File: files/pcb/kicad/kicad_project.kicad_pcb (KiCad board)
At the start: 2 copper layers, 100 x 102 mm, 115 parts, among them CON1 USB_MINI_B, IC1 ATMEGA328-A, IC10 FET, IC11 DS1307, IC12 LPS331AP, IC13 AM2321, IC2 IC_16PIN, IC3 IC_4PIN, IC4 IC_4PIN, IC5 SN74141_K155NA, IC6 TLP627-4, IC7 TLP627-4, IC8 MY_3_TERMINAL_REGULATOR, IC9 ICM7555CD, K1 CONN_3, K2 CONN_3, K3 CONN_3, K4 CONN_3, P1 CONN_6, SW1 SW_PUSH, SW2 EVQWK, SW3 SW_PUSH, SW4 SW_PUSH, SW5 SW_PUSH, T1 2SC, T2 2SC, T3 2SA, U1 NEON, U10 NIXIE_IN_16, U11 DC_JACK, U12 LOAD, U13 remocon, U14 napion, U15 MY_PIN52, U16 MY_PIN52, U17 MY_PIN52, U18 MY_PIN52, U2 NEON, U3 NEON, U4 NEON, U5 NIXIE_IN_16, U6 NIXIE_IN_16, U7 NIXIE_IN_16, U8 NIXIE_IN_16, U9 NIXIE_IN_16, X1 12MHz, X2 32.768kHz

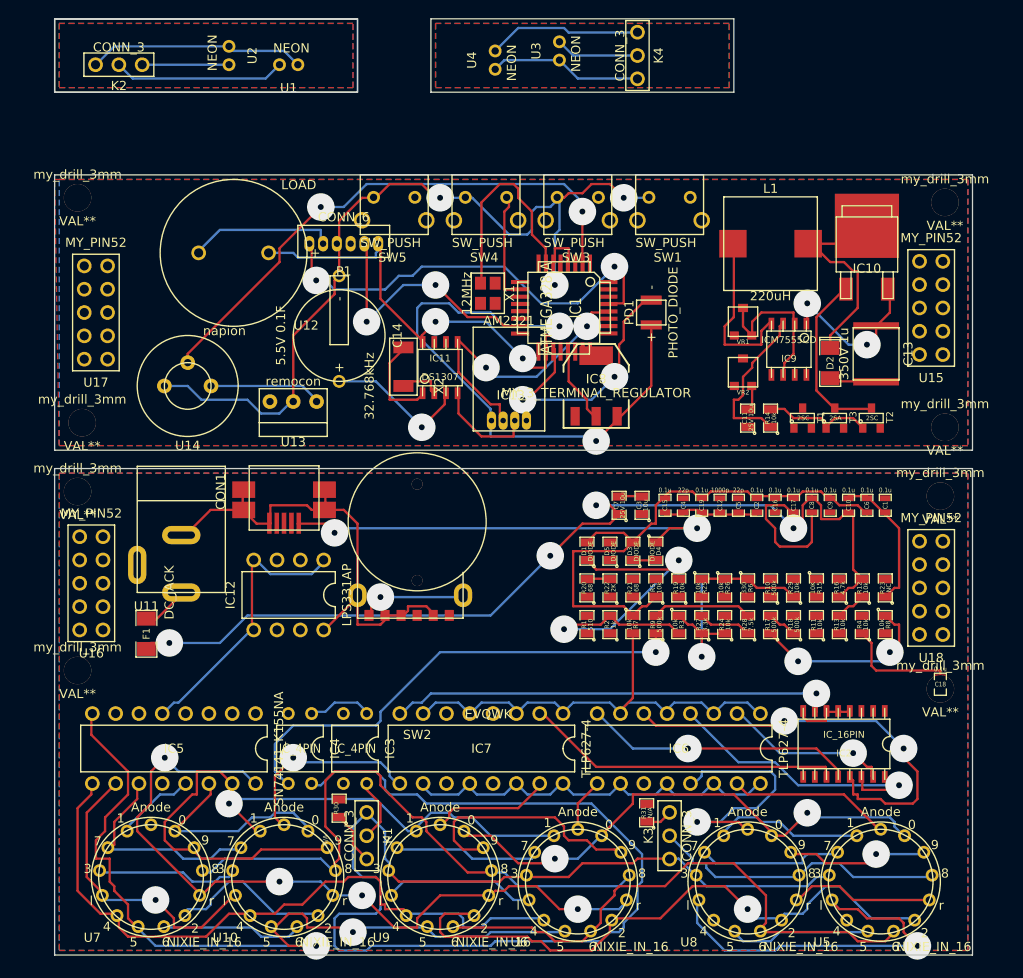
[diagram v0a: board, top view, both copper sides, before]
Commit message: PCB
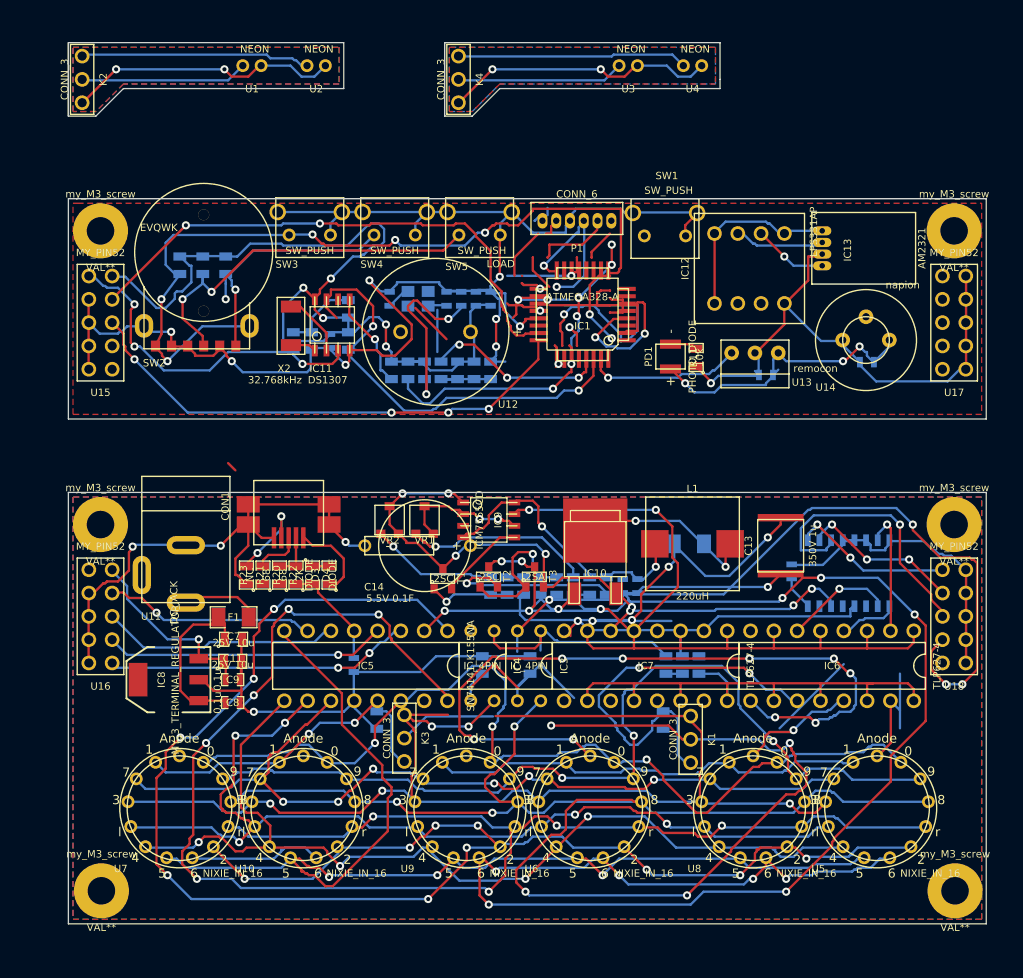
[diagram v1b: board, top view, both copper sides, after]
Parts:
- removed my_drill_3mm (x8): VAL**, my_drill_3mm
- added my_M3_screw: VAL**, my_M3_screw, F.Cu at (257.6, 181.5)
- added my_M3_screw: VAL**, my_M3_screw, F.Cu at (257.5, 109.6)
- added my_M3_screw: VAL**, my_M3_screw, F.Cu at (164.5, 109.6)
- added my_M3_screw: VAL**, my_M3_screw, F.Cu at (164.6, 181.5)
- added my_M3_screw: VAL**, my_M3_screw, F.Cu at (164.5, 141.6)
- added my_M3_screw: VAL**, my_M3_screw, F.Cu at (257.5, 141.6)
- C1, C10, C12, C15, C16, C17, C18, C19, C2, C3, C4, C5, C6, D1, D2, D5, IC2, R1, R10, R12, R13, R14, R15, R16, R17, R18, R19, R2, R24, R25, R26, R27, R28, R29, R3, R30, R31, R4, R5, R6, R7, R8, R9, X1: moved to B.Cu
- IC12: footprint my_dip8 -> my_dip_module
- moved U17 93.5 mm to (257.5, 119.6)
- moved U15 90.5 mm to (164.5, 119.6)
- moved C18 76.3 mm to (189.5, 121.6)
- moved U14 74.1 mm to (247.9, 121.5)
- moved R24 71.1 mm to (173.1, 113.3), turned to 270 degrees
- moved R23 69.6 mm to (180.4, 147.1)
- moved C9 67.8 mm to (178.9, 158.5), turned to 0 degrees
- moved R26 66.8 mm to (175.6, 113.3)
- moved C8 66.7 mm to (178.9, 161.0), turned to 0 degrees
- moved R25 62.6 mm to (178.1, 113.3)
- moved C11 62.0 mm to (178.9, 156.5), turned to 0 degrees
- moved IC12 60.8 mm to (235.2, 113.7), turned to 270 degrees
- moved R4 56.7 mm to (198.0, 124.8), turned to 270 degrees
- moved R28 56.7 mm to (187.5, 121.6), turned to 270 degrees
- moved IC8 56.5 mm to (171.9, 158.5), turned to 90 degrees
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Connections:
- C10 pad 1: GND -> GND_L
- C11 pad 1: +5V -> 5V_L
- C11 pad 2: GND -> GND_L
- C12 pad 2: GND -> GND_L
- C13 pad 2: GND -> GND_L
- C14 pad 1: N-00000113 -> CLK_PW_L
- C15 pad 2: GND -> GND_L
- C6 pad 1: GND -> GND_L
- C7 pad 2: GND -> GND_L
- C8 pad 2: GND -> GND_L
- C9 pad 1: +5V -> 5V_L
- C9 pad 2: GND -> GND_L
- D5 pad 2: N-00000113 -> CLK_PW_H
- IC10 pad 3: GND -> GND_L
- IC11 pad 3: N-00000113 -> CLK_PW_H
- IC2 pad 1: /PB0 -> /PB_P0
- IC2 pad 10: N-0000074 -> /nixie/L3
- IC2 pad 11: N-0000073 -> /nixie/L4
- IC2 pad 12: N-0000069 -> /nixie/L5
- IC2 pad 13: N-0000072 -> /nixie/L6
- IC2 pad 14: N-0000071 -> /nixie/L7
- IC2 pad 15: N-0000070 -> /nixie/L8
- IC2 pad 2: /PB1 -> /PB_P1
- IC2 pad 3: /PB2 -> /PB_P2
- IC2 pad 4: GND -> GND_L
- IC2 pad 5: GND -> GND_L
- IC2 pad 6: GND -> GND_L
- IC2 pad 7: N-0000068 -> /nixie/L1
- IC2 pad 8: GND -> GND_L
- IC2 pad 9: N-0000075 -> /nixie/L2
- IC3 pad 2: /MOSI -> /PB_P3
- IC4 pad 2: /MISO -> /PB_P4
- IC5 pad 12: GND -> GND_L
- IC5 pad 3: /PC3 -> /PC_P3
- IC5 pad 4: /PC2 -> /PC_P2
- IC5 pad 6: /PC1 -> /PC_P1
- IC5 pad 7: /PC0 -> /PC_P0
- IC6 pad 2: N-0000070 -> /nixie/L1
- IC6 pad 4: N-0000071 -> /nixie/L2
- IC6 pad 6: N-0000072 -> /nixie/L3
- IC6 pad 8: N-0000069 -> /nixie/L4
- IC7 pad 2: N-0000073 -> /nixie/L5
- IC7 pad 4: N-0000074 -> /nixie/L6
- IC7 pad 6: N-0000075 -> /nixie/L7
- IC7 pad 8: N-0000068 -> /nixie/L8
- IC8 pad 2: GND -> GND_L
- IC8 pad 3: +5V -> 5V_L
- IC9 pad 1: GND -> GND_L
- R10 pad 2: GND -> GND_L
- R27 pad 1: +5V -> 5V_L
- R30 pad 2: GND -> GND_L
- R31 pad 2: GND -> GND_L
- R9 pad 2: GND -> GND_L
- T1 pad 3: GND -> GND_L
- T3 pad 2: GND -> GND_L
- U11 pad 3: GND -> GND_L
- U15 pad 1: (no net) -> CLK_PW_H
- U15 pad 10: (no net) -> +5V
- U15 pad 2: (no net) -> GND
- U15 pad 3: (no net) -> GND
- U15 pad 4: (no net) -> GND
- U15 pad 5: (no net) -> GND
- U15 pad 6: (no net) -> /PC3
- U15 pad 7: (no net) -> /PC2
- U15 pad 8: (no net) -> /PC1
- U15 pad 9: (no net) -> /PC0
- U16 pad 1: (no net) -> CLK_PW_L
- U16 pad 10: (no net) -> 5V_L
- U16 pad 2: (no net) -> GND_L
- U16 pad 3: (no net) -> GND_L
- U16 pad 4: (no net) -> GND_L
- U16 pad 5: (no net) -> GND_L
- U16 pad 6: (no net) -> /PC_P3
- U16 pad 7: (no net) -> /PC_P2
- U16 pad 8: (no net) -> /PC_P1
- U16 pad 9: (no net) -> /PC_P0
- U17 pad 1: (no net) -> /PB0
- U17 pad 10: (no net) -> GND
- U17 pad 2: (no net) -> /PB1
- U17 pad 3: (no net) -> /PB2
- U17 pad 4: (no net) -> /MOSI
- U17 pad 5: (no net) -> /MISO
- U17 pad 6: (no net) -> GND
- U17 pad 7: (no net) -> GND
- U17 pad 8: (no net) -> GND
- U17 pad 9: (no net) -> GND
- U18 pad 1: (no net) -> /PB_P0
- U18 pad 10: (no net) -> GND_L
- U18 pad 2: (no net) -> /PB_P1
- U18 pad 3: (no net) -> /PB_P2
- U18 pad 4: (no net) -> /PB_P3
- U18 pad 5: (no net) -> /PB_P4
- U18 pad 6: (no net) -> GND_L
- U18 pad 7: (no net) -> GND_L
- U18 pad 8: (no net) -> GND_L
- U18 pad 9: (no net) -> GND_L
- VR2 pad 2: GND -> GND_L
- VR2 pad 3: GND -> GND_L
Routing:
- net GND_L: track 0.00 -> 192.4 mm, vias 0 -> 8
- net /nixie/N0: track 76.5 -> 199.0 mm, vias 0 -> 10
- net /nixie/N1: track 85.5 -> 184.7 mm, vias 1 -> 13
- net (no net): track 0.00 -> 95.3 mm, vias 0 -> 3
- net /nixie/Sheet53F9F7BA/dot_cathode_l: track 107.9 -> 197.8 mm, vias 0 -> 7
- net /Sheet53F8FD69/A: track 11.9 -> 96.7 mm, vias 1 -> 7
- net /nixie/N2: track 100.4 -> 180.0 mm, vias 4 -> 9
- net /nixie/Sheet53F9F7BA/3: track 5.85 -> 81.7 mm, vias 0 -> 9
- net +5V: track 264.3 -> 190.2 mm, vias 5 -> 11
- net N-0000078: track 124.6 -> 50.9 mm, vias 4 -> 2
- net /PB_P3: track 0.00 -> 62.9 mm, vias 0 -> 3
- net /PC0: track 0.00 -> 59.3 mm, vias 0 -> 2
- net N-0000055: track 55.6 -> 112.0 mm, vias 0 -> 3
- net /PC1: track 0.00 -> 55.9 mm, vias 0 -> 4
- net N-0000063: track 53.6 -> 3.47 mm, vias 1 -> 0
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- removed copper zone on B.Cu, net N-00000101
- removed copper zone on F.Cu, net N-00000101
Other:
- board size 100 x 102 mm -> 100 x 96 mm
